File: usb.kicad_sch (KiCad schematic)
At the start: 15 parts, among them J11 USB_C_Receptacle_USB2.0_16P, SW3 SW_Rotary_1x3_MP, SW4 SW_Rotary_1x3_MP

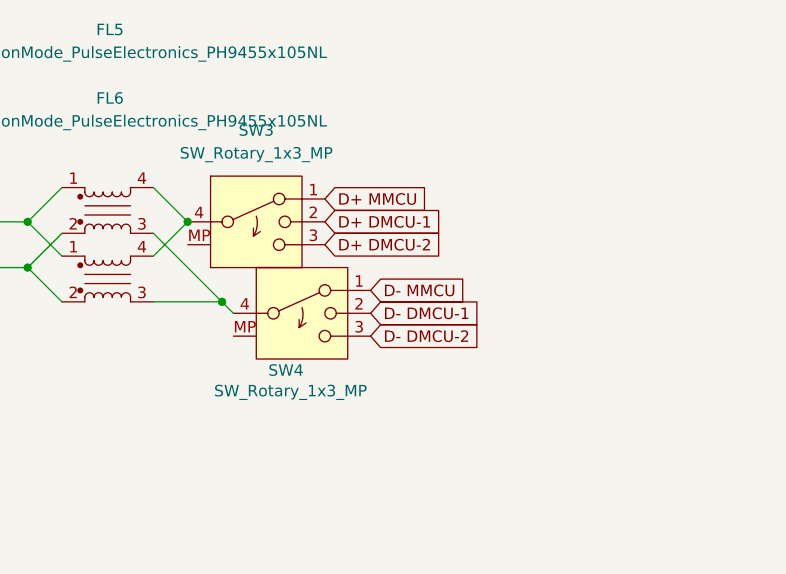
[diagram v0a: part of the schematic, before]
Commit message: misc fixes
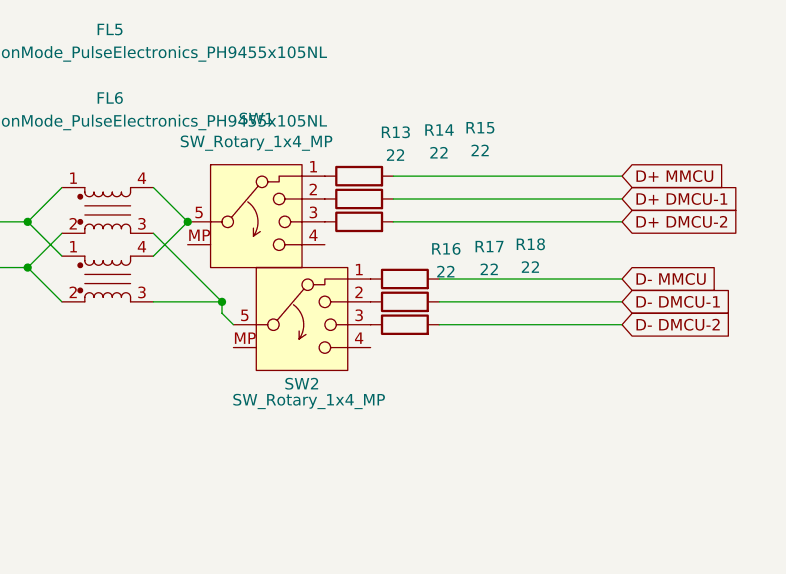
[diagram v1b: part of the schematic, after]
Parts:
- removed SW3, SW4: SW_Rotary_1x3_MP, symbol Switch:SW_Rotary_1x3_MP
- added R13, R14, R15, R16, R17, R18: 22, symbol Device:R
- added SW1, SW2: SW_Rotary_1x4_MP, symbol Switch:SW_Rotary_1x4_MP
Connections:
- net D+ DMCU-1: now also R14.2
- net D+ DMCU-2: now also R15.2
- net D+ MMCU: now also R13.2
- net D- DMCU-1: now also R17.2
- net D- DMCU-2: now also R18.2
- net D- MMCU: now also R16.2
- net at FL5.4, FL6.4: now also SW1.5
- net at FL5.3, FL6.3: now also SW2.5
- new net: R17.1, SW2.2
- new net: R16.1, SW2.1
- new net: R18.1, SW2.3
- new net: R15.1, SW1.3
- new net: R13.1, SW1.1
- new net: R14.1, SW1.2
